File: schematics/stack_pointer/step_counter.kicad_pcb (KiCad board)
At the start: 2 copper layers, 100 x 91 mm, 17 parts, among them U1 74HC00, U2 74HC193, U3 74HC193, U4 74HC193, U5 74HC193, U6 74HC245, U7 74HC245

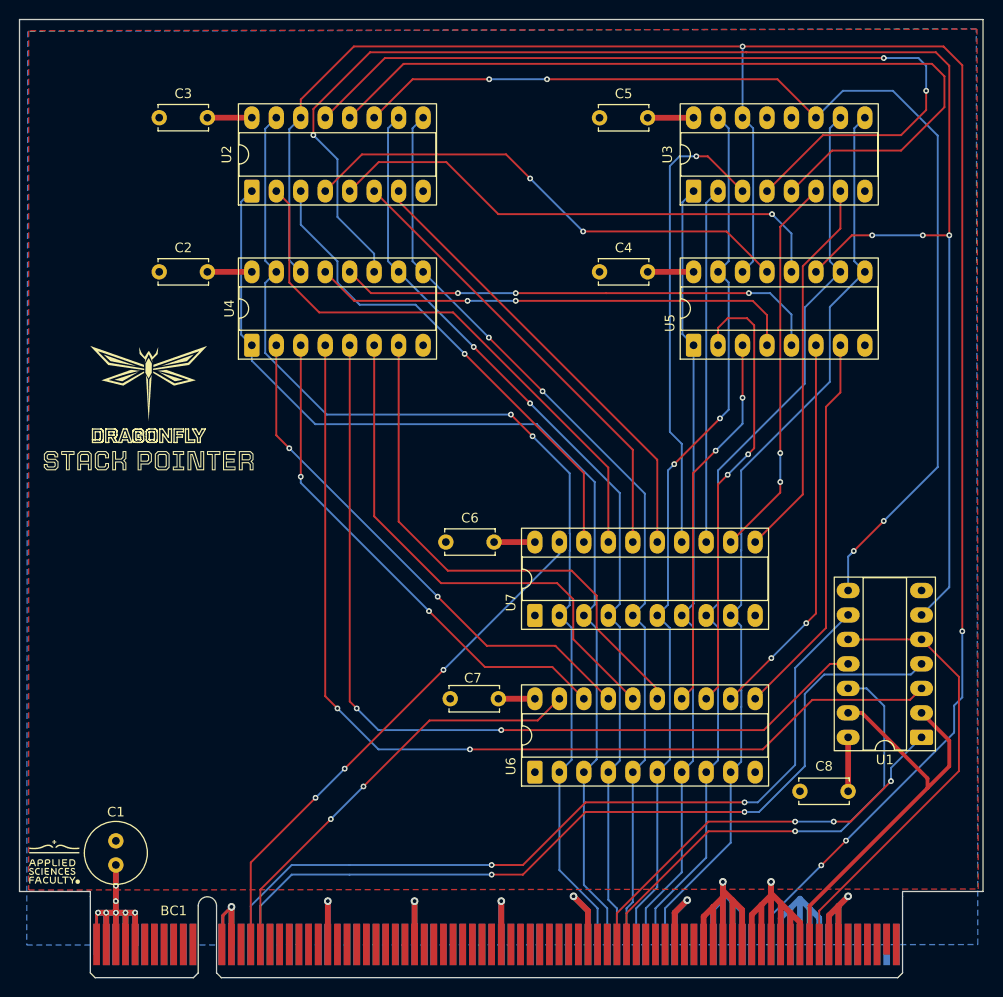
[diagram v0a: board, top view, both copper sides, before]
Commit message: update pc and sp
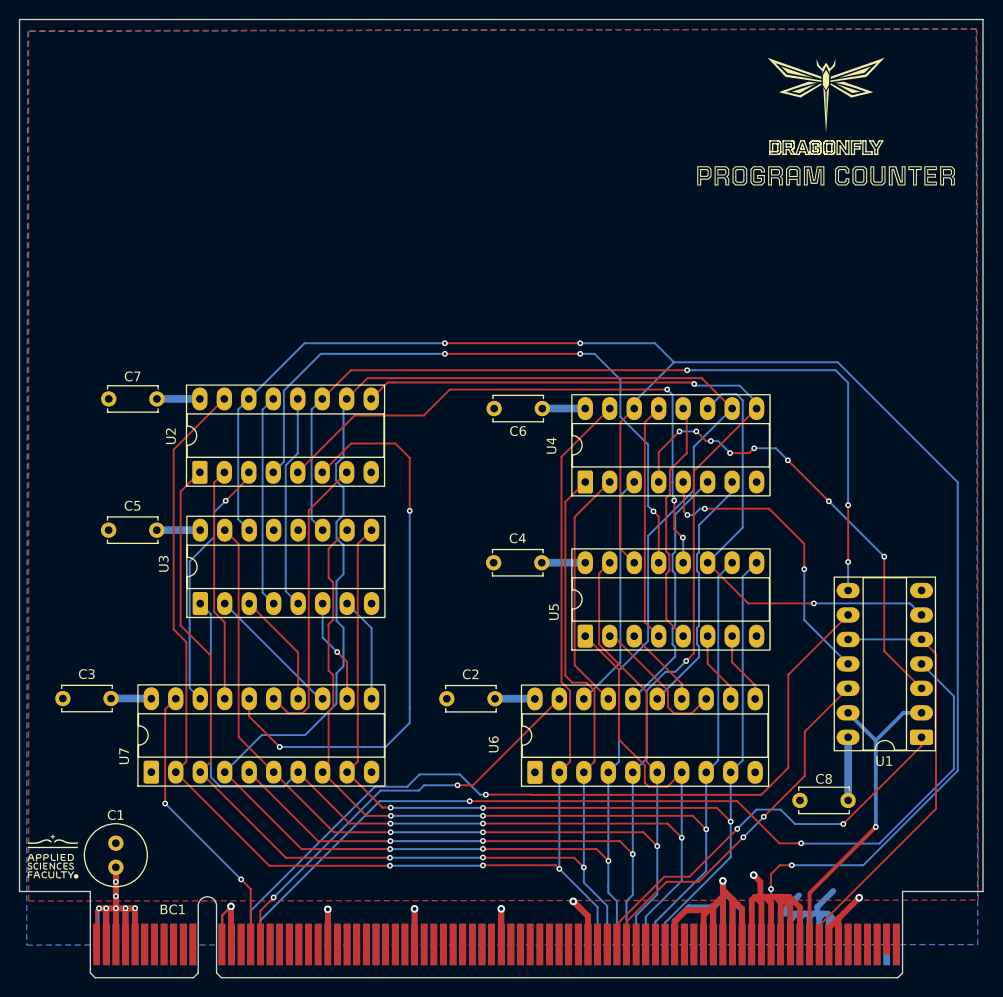
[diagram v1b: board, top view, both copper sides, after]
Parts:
- removed kibuzzard-6911C575: G***, kibuzzard-6911C575
- added kibuzzard-6911BE41: G***, kibuzzard-6911BE41, F.Cu at (190.2, 50.2)
- moved U3 66.7 mm to (125.3, 94.6)
- moved C5 66.5 mm to (115.8, 87.0)
- moved C3 61.1 mm to (111.0, 104.5)
- moved C2 53.4 mm to (150.8, 104.5)
- moved C7 47.2 mm to (120.8, 73.4)
- moved U7 43.0 mm to (120.2, 112.1)
- moved U4 37.4 mm to (165.2, 82.0)
- moved U5 32.2 mm to (165.2, 98.0)
- moved C4 32.1 mm to (155.7, 90.4)
- moved U2 29.7 mm to (125.2, 81.0)
- moved C6 14.7 mm to (155.8, 74.4)
- moved C8 0.95 mm to (192.5, 115.0)
- moved C1 0.24 mm to (116.5, 122.0)
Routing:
- net /Pl: track 162.2 -> 47.3 mm, vias 4 -> 1
- net /DATA2: track 98.1 -> 195.9 mm, vias 2 -> 3
- net Net-(U2-~{BO}): track 89.9 -> 22.2 mm, vias 2 -> 0
- net Net-(U2-~{CO}): track 87.3 -> 22.3 mm
- net /CPu: track 92.8 -> 31.9 mm, vias 2 -> 3
- net /CPd: track 103.2 -> 48.5 mm, vias 2 -> 8
- net /DATA3: track 98.1 -> 147.4 mm, vias 2 -> 5
- net /DH4: track 49.0 -> 12.0 mm, vias 1 -> 0
- net /DH1: track 58.8 -> 24.4 mm
- net /RESET: track 214.4 -> 181.3 mm
- net /DL6: track 40.4 -> 7.51 mm, vias 2 -> 0
- net /DL7: track 40.4 -> 7.51 mm
- net /DL5: track 47.1 -> 15.0 mm, vias 2 -> 0
- net /DATA0: track 114.7 -> 146.1 mm, vias 2 -> 3
- net /DATA5: track 82.2 -> 113.0 mm, vias 0 -> 3
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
